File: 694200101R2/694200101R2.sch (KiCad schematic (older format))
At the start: 264 parts, among them J1 USB_C_Receptacle_USB2.0, J2 Conn_01x06_Male, J3 Conn_01x02_Male, SW1 MX_SW, SW10 MX_SW, SW100 MX_SW, SW101 MX_SW, SW102 MX_SW, SW103 MX_SW, SW104 MX_SW, SW105 MX_SW, SW106 MX_SW, SW107 MX_SW, SW108 SW_SPST, SW109 SW_SPDT, SW11 MX_SW, SW12 MX_SW, SW13 MX_SW, SW14 MX_SW, SW15 MX_SW, SW16 MX_SW, SW17 MX_SW, SW18 MX_SW, SW19 MX_SW, SW2 MX_SW, SW20 MX_SW, SW21 MX_SW, SW22 MX_SW, SW23 MX_SW, SW24 MX_SW, SW25 MX_SW, SW26 MX_SW, SW27 MX_SW, SW28 MX_SW, SW29 MX_SW, SW3 MX_SW, SW30 MX_SW, SW31 MX_SW, SW32 MX_SW, SW33 MX_SW, SW34 MX_SW, SW35 MX_SW, SW36 MX_SW, SW37 MX_SW, SW38 MX_SW, SW39 MX_SW, SW4 MX_SW, SW40 MX_SW, SW41 MX_SW, SW42 MX_SW, SW43 MX_SW, SW44 MX_SW, SW45 MX_SW, SW46 MX_SW, SW47 MX_SW, SW48 MX_SW, SW49 MX_SW, SW5 MX_SW, SW50 MX_SW, SW51 MX_SW, SW52 MX_SW, SW53 MX_SW, SW54 MX_SW, SW55 MX_SW, SW56 MX_SW, SW57 MX_SW, SW58 MX_SW, SW59 MX_SW, SW6 MX_SW, SW60 MX_SW, SW61 MX_SW, SW62 MX_SW, SW63 MX_SW, SW64 MX_SW, SW65 MX_SW, SW66 MX_SW, SW67 MX_SW, SW68 MX_SW, SW69 MX_SW, SW7 MX_SW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

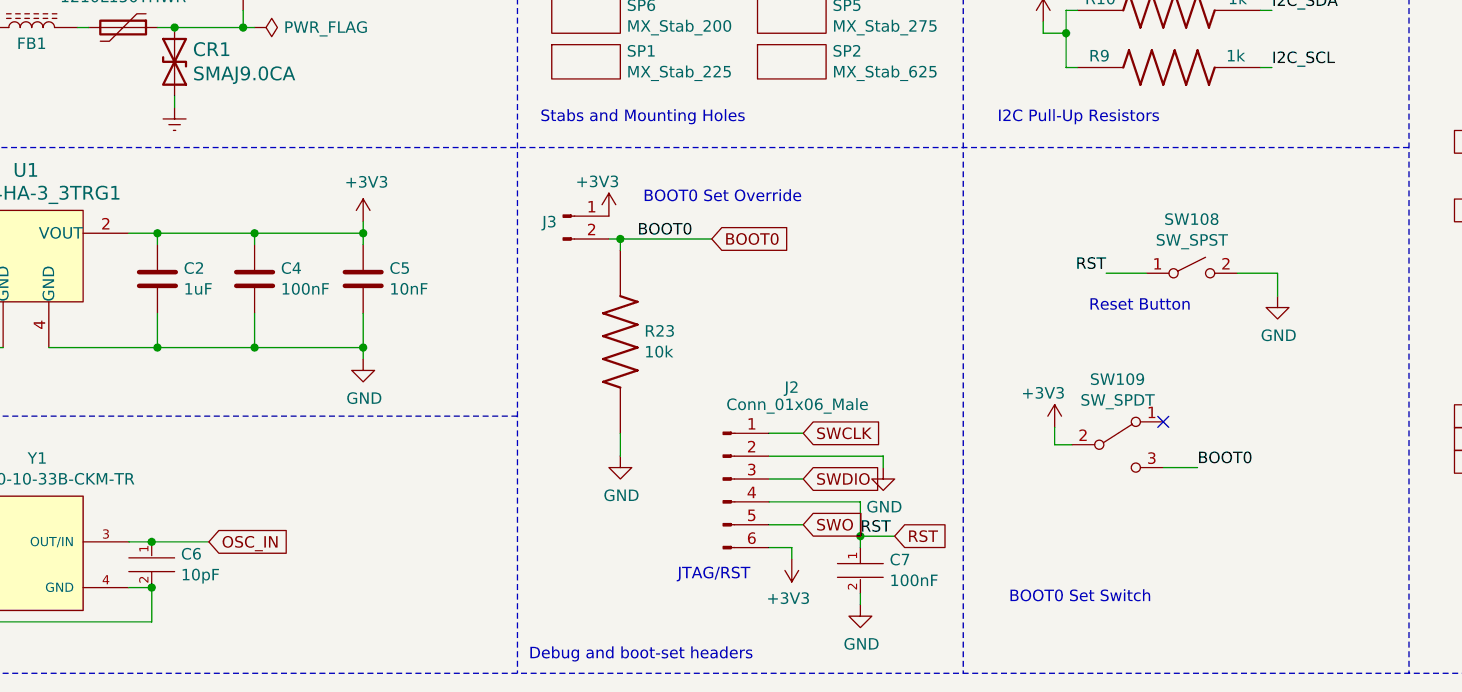
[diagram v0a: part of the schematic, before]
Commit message: sch review
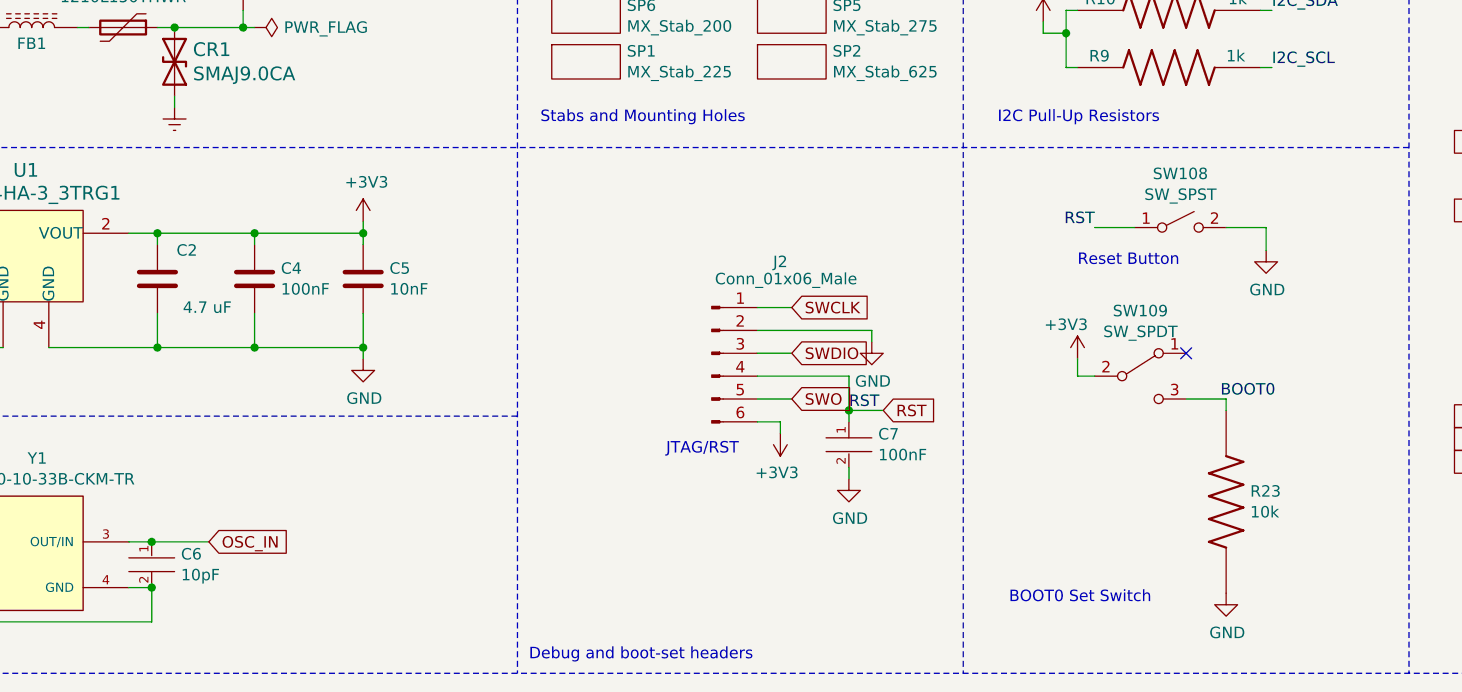
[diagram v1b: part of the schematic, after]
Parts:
- removed J3: Conn_01x02_Male, Connector_PinHeader_2.54mm:PinHeader_1x02_P2.54mm_Vertical, symbol Connector:Conn_01x02_Male
- C2: value 1uF -> 4.7 uF; footprint Capacitor_SMD:C_0603_1608Metric -> Capacitor_SMD:C_0805_2012Metric
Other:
- note removed: "BOOT0 Set Override"
- moved on the sheet: C7, J2, R23, SW108, SW109
